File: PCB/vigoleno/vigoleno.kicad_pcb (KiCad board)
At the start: 6 copper layers, 80.8 x 50 mm, 181 parts, among them J1 9P-MSD-PP-V2, J3 USB_OTG, J4 IPEX RF Coaxial Connector SMD, M1 MODULE_RTL8188, U1 MT29F8G08ABABA, U2 ISL8022, U3 ALLWINNER-A13(176-LQFP), U4 TLV62569-SOT23-6, U5 TPS62233DRYR, U6 AS4C256M16D3A-12BAN(96-FBGA), U7 MCP130T-300ITT, Y1 Crystal_GND24_24MHz

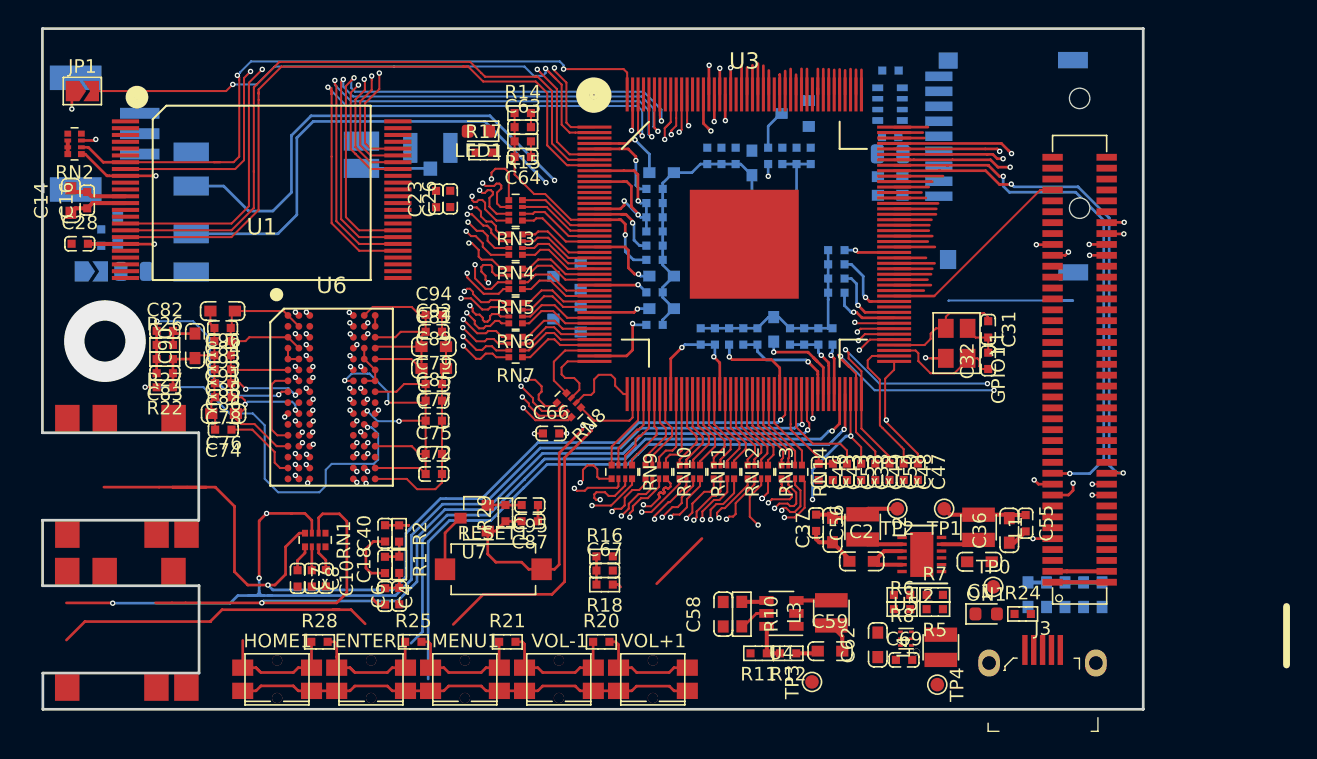
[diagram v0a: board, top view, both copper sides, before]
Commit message: update March 6 2019
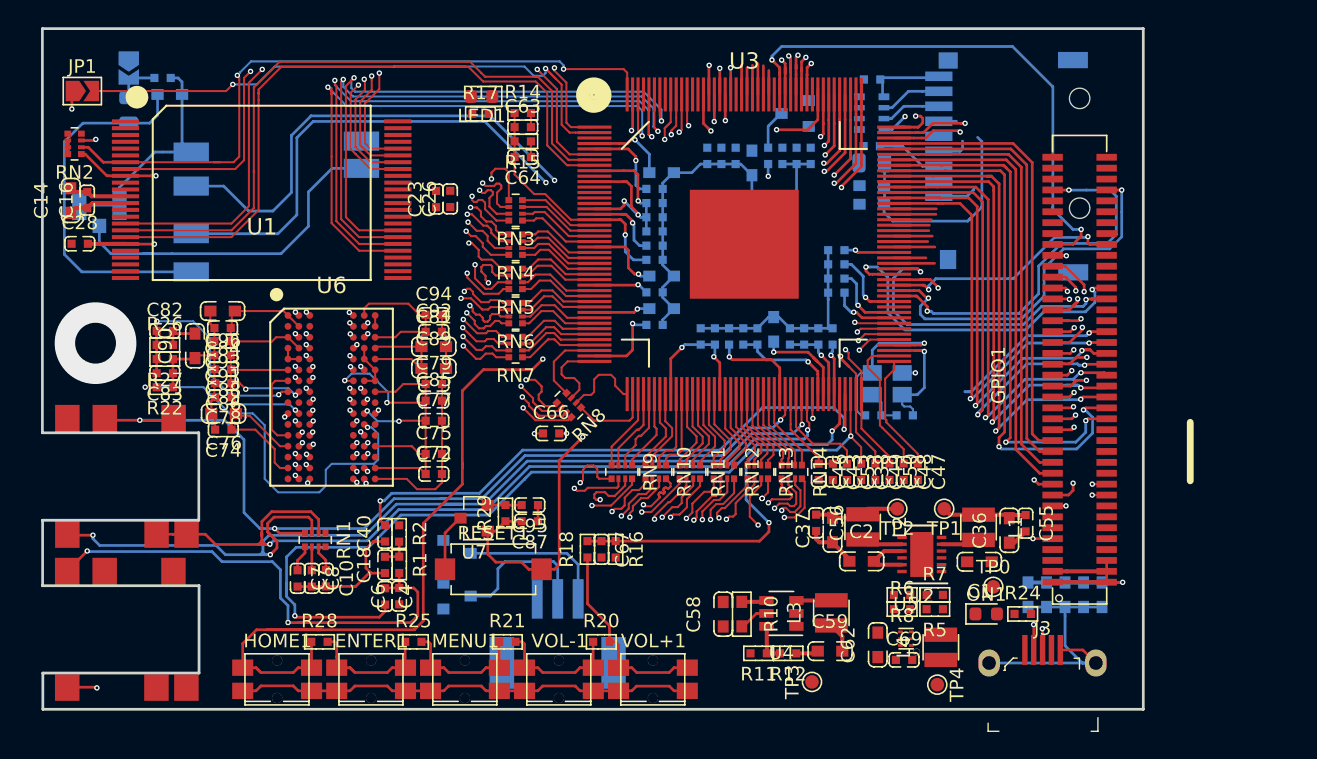
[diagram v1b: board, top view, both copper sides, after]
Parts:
- C31, C32, Y1: moved to B.Cu
- moved DEBUG1 49.6 mm to (589.9, -415.9), turned to 180 degrees
- moved D3 24.8 mm to (582.5, -418.7), turned to 0 degrees
- moved J4 24.7 mm to (556.2, -446.9)
- moved D2 19.0 mm to (582.5, -421.9), turned to 0 degrees
- moved JP2 15.2 mm to (558.4, -457.5), turned to 270 degrees
- moved C97 12.6 mm to (560.9, -456.8), turned to 180 degrees
- moved L6 11.8 mm to (558.4, -454.4), turned to 270 degrees
- moved C98 10.7 mm to (561.4, -455.6), turned to 180 degrees
- moved C31 10.5 mm to (613.0, -432.0), turned to 0 degrees
- moved C32 7.32 mm to (615.4, -432.0), turned to 180 degrees
- moved Y1 5.92 mm to (614.1, -434.3), turned to 0 degrees
- moved R18 2.88 mm to (592.1, -422.2), turned to 90 degrees
- moved R17 2.86 mm to (584.2, -454.1)
- moved LED1 2.56 mm to (584.3, -455.4)
- moved C67 1.57 mm to (593.1, -422.2), turned to 270 degrees
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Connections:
- GPIO1 pad 10: /PIN39_USBH-EN -> /TWI2-SCK
- GPIO1 pad 11: /PIN38_VGA-DIS -> /USB0-IDDET
- GPIO1 pad 12: /PIN37_LED1 -> /TWI2-SDA
- GPIO1 pad 13: /PIN15_NCE1 -> /SPI2-MOSI
- GPIO1 pad 14: /USB0-DRV -> /SPI2-CS0
- GPIO1 pad 15: /USB0-VBUSDET -> /SPI2-MISO
- GPIO1 pad 16: /USB0-IDDET -> /SPI2-CLK
- GPIO1 pad 21: /PIN36 -> /LCD-VSYNC
- GPIO1 pad 22: /PIN35 -> /USB0-VBUSDET
- GPIO1 pad 23: /PIN34 -> /LCD-HSYNC
- GPIO1 pad 24: /PIN33 -> /USB0-DRV
- GPIO1 pad 25: /PIN32 -> /LCD-DE
- GPIO1 pad 26: /PIN31 -> /PIN39_USBH-EN
- GPIO1 pad 27: /PIN28_NDQS -> /LCD-CLK
- GPIO1 pad 28: /PIN19_NRB1 -> /PIN38_VGA-DIS
- GPIO1 pad 29: /PIN30 -> /LCD-D23
- GPIO1 pad 30: /PIN29 -> /PIN37_LED1
- GPIO1 pad 31: /SPI2-MISO -> /LCD-D22
- GPIO1 pad 32: /SPI2-MOSI -> /PIN36
- GPIO1 pad 33: /SPI2-CLK -> /LCD-D21
- GPIO1 pad 34: /SPI2-CS0 -> /PIN35
- GPIO1 pad 35: /PIN11_TWI1-SDA -> /LCD-D20
- GPIO1 pad 36: /TWI2-SCK -> /PIN34
- GPIO1 pad 37: /PIN10_TWI1-SCK -> /LCD-D19
- GPIO1 pad 38: /TWI2-SDA -> /PIN33
- GPIO1 pad 39: /PIN8 -> /LCD-D18
- GPIO1 pad 40: /PIN9 -> /PIN32
- GPIO1 pad 41: /PIN6_PWM0 -> /LCD-D15
- GPIO1 pad 42: /PIN7 -> /PIN31
- GPIO1 pad 43: /LCD-D23 -> /LCD-D14
- GPIO1 pad 44: /LCD-D22 -> /PIN30
- GPIO1 pad 45: /LCD-D21 -> /LCD-D13
- GPIO1 pad 46: /LCD-D20 -> /PIN29
- GPIO1 pad 47: /LCD-D19 -> /LCD-D12
- GPIO1 pad 48: /LCD-D18 -> /PIN28_NDQS
- GPIO1 pad 49: /LCD-D15 -> /LCD-D11
- GPIO1 pad 50: /LCD-D14 -> /PIN19_NRB1
- GPIO1 pad 51: /LCD-D13 -> /LCD-D10
- GPIO1 pad 52: /LCD-D12 -> /PIN15_NCE1
- GPIO1 pad 53: /LCD-D11 -> /LCD-D7
- GPIO1 pad 54: /LCD-D10 -> /PIN11_TWI1-SDA
- GPIO1 pad 56: /LCD-D7 -> /PIN10_TWI1-SCK
- GPIO1 pad 57: /LCD-D4 -> /LCD-D5
- GPIO1 pad 58: /LCD-D5 -> /PIN9
- GPIO1 pad 59: /LCD-D2 -> /LCD-D4
- GPIO1 pad 60: /LCD-D3 -> /PIN8
- GPIO1 pad 61: /LCD-HSYNC -> /LCD-D3
- GPIO1 pad 62: /LCD-VSYNC -> /PIN7
- GPIO1 pad 63: /LCD-CLK -> /LCD-D2
- GPIO1 pad 64: /LCD-DE -> /PIN6_PWM0
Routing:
- net /TPX2: track 59.8 -> 9.97 mm, vias 3 -> 1
- net /LCD-D19: track 1.81 -> 50.7 mm, vias 0 -> 2
- net /TPY2: track 58.3 -> 9.81 mm, vias 3 -> 1
- net /LCD-D10: track 2.32 -> 49.0 mm, vias 0 -> 2
- net /LCD-D15: track 1.77 -> 48.4 mm, vias 0 -> 2
- net /LCD-D20: track 1.81 -> 47.6 mm, vias 0 -> 2
- net /LCD-D18: track 1.86 -> 45.9 mm, vias 0 -> 2
- net /LCD-D13: track 1.80 -> 45.7 mm, vias 0 -> 2
- net /LCD-D14: track 1.84 -> 45.5 mm, vias 0 -> 2
- net /LCD-D4: track 1.87 -> 44.0 mm, vias 0 -> 2
- net /LCD-D11: track 1.86 -> 43.7 mm, vias 0 -> 2
- net /LCD-D12: track 1.85 -> 43.5 mm, vias 0 -> 2
- net /LCD-D5: track 1.45 -> 40.5 mm, vias 0 -> 2
- net /LCD-D2: track 1.45 -> 40.0 mm, vias 0 -> 2
- net /LCD-D3: track 1.72 -> 39.8 mm, vias 0 -> 2
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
